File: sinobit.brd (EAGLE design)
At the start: 92 x 92.1 mm, 254 parts, among them J1 TWIG_2.0, J2 TWIG_2.0, U1 SPX3819, U10 16MHZ2520, U6 IC_NRF51822_MODULE, U8 HT1632C_QFP52, U9 16MHZ2520

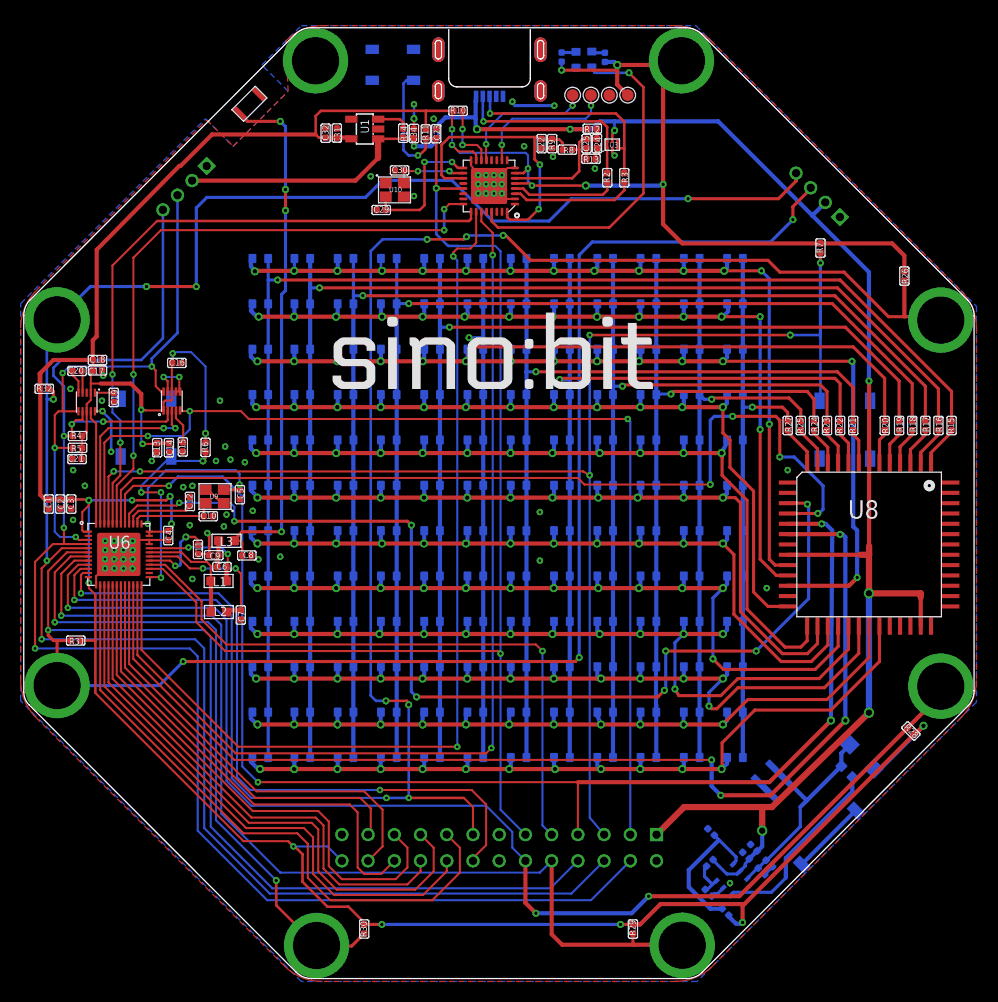
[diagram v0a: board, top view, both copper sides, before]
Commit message: sinobit-V1.0
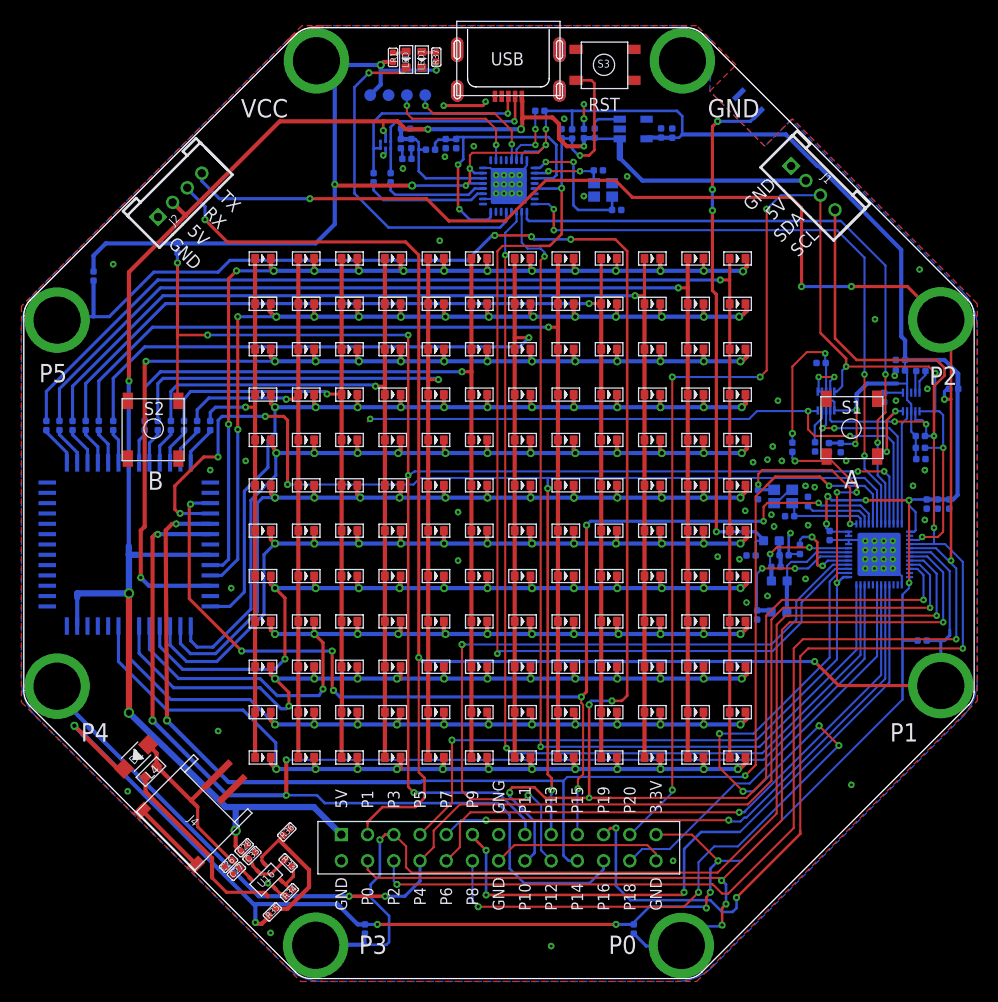
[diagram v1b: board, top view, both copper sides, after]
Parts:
- removed U$1: (no value), Logo:SINOBIT3
- removed U$13: IC_MMA8653FCR1, mirco：bit:MMA8653FC
- removed U$4: PS7516, microbit2:PS7516
- removed U$6: TIANXIAN, microbit2:TIANXIAN
- removed U$7: IC_MKL26Z128VFM4, Modulebit_open_Eagle:MKL26Z168VFM4
- added E$1: (no value), XZX1:文字
- added E$2: (no value), XZX:SINOBIT2
- added E$3: (no value), XZX1:ELECEOW
- added E$4: (no value), XZX:SINOBIT编号
- added E$5: (no value), XZX:XXX
- added U11: TIANXIAN, microbit2:TIANXIAN
- added U12: IC_MKL26Z128VFM4, Modulebit_open_Eagle:MKL26Z168VFM4
- added U14: IC_MMA8653FCR1, mirco：bit:MMA8653FC
- added U16: PS7516, microbit2:PS7516
- C33: value 22uF -> 10uF
- R26, R28, R29, R30, R31, R32: value 3.3M -> 2M
- R33: value 525K -> 510k
- moved R32 88.1 mm to (77.4, 30.1), flipped to the bottom
- moved R15 87.7 mm to (-10.5, 26.5), flipped to the bottom
- moved C1 87.2 mm to (77.0, 18.9), flipped to the bottom
- moved U$35 85.6 mm to (76.2, 1.36), flipped to the bottom
- moved U$39 85.6 mm to (76.2, 36.8), flipped to the bottom
- moved U$48 85.6 mm to (-9.42, 36.8), flipped to the bottom
- moved U$49 85.6 mm to (-9.42, 1.30), flipped to the bottom
- moved R16 85.1 mm to (-9.19, 26.5), flipped to the bottom
- moved C2 85.0 mm to (75.9, 18.9), flipped to the bottom
- moved C3 82.9 mm to (74.8, 18.9), flipped to the bottom
- moved R17 82.6 mm to (-7.92, 26.5), flipped to the bottom
- moved R31 82.0 mm to (74.4, 5.71), flipped to the bottom
- moved C20 81.7 mm to (74.2, 31.8), flipped to the bottom
- moved C21 81.7 mm to (74.2, 23.3), flipped to the bottom
- moved R4 81.6 mm to (74.2, 25.5), flipped to the bottom
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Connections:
- removed net N$7: R30.2, U$51.P$1, U6.7
- removed net P0.8: U$12.P$9, U6.14
- new net P0.3: R30.2, U$12.P$25, U$51.P$1, U6.7
- net 3.3V: now also U$12.P$13, U12.15, U12.5, U12.7, U14.8, U14.P1; no longer U$12.P$14, U$13.8, U$13.P1, U$7.15, U$7.5, U$7.7
- net 8653_INT1: now also U14.P3; no longer U$13.P3
- net 8653_INT2: now also U14.P5; no longer U$12.P$2, U$13.P5
- net BTN_A: now also U$12.P$4
- net BTN_B: now also U$12.P$8; no longer U$12.P$3
- net GND: now also U$12.P$14, U12.16, U12.2, U12.8, U14.6, U14.7, U14.9, U16.P2; no longer U$12.P$13, U$13.6, U$13.7, U$13.9, U$4.P2, U$7.16, U$7.2, U$7.8
- net MISO: now also U$12.P$17; no longer U$12.P$4
- net MOSI: now also U$12.P$10
- net N$11: now also U12.29; no longer U$7.29
- net N$14: now also U12.3; no longer U$7.3
- net N$15: now also U12.4; no longer U$7.4
- net N$16: now also U12.17; no longer U$7.17
- net N$17: now also U12.18; no longer U$7.18
- net N$18: now also U16.P4; no longer U$4.P4
- net N$19: now also U16.P6; no longer U$4.P6
- net N$22: now also U16.P1; no longer U$4.P1
- net N$23: now also U11.P$1; no longer U$6.P$1
- net N$26: now also U16.P3; no longer U$4.P3
- net N$3: now also U12.14; no longer U$7.14
- net N$4: now also U14.P4; no longer U$13.P4
- net N$8: now also U12.10; no longer U$7.10
- net N$9: now also U12.13; no longer U$7.13
- net P0.10: now also U$12.P$6; no longer U$12.P$10
- net P0.11: now also U$12.P$5; no longer U$12.P$17
- net P0.12: now also U$12.P$22; no longer U$12.P$11
- net P0.13: now also U$12.P$15; no longer U$12.P$16
- net P0.14: no longer U$12.P$12
- net P0.15: no longer U$12.P$15
- net P0.16: now also U$12.P$16
- net P0.18: now also U$12.P$21
- net P0.2/RX: now also U$12.P$2; no longer U$12.P$23
- net P0.20: now also U$12.P$18; no longer U$12.P$5
- net P0.4: now also U$12.P$3; no longer U$12.P$22
- net P0.5: now also U$12.P$23; no longer U$12.P$21
- net P0.6: now also U$12.P$19; no longer U$12.P$8
- net P0.7: no longer U$12.P$19
- net P0.9: no longer U$12.P$18
- net RST: now also U12.19, U12.32; no longer U$7.19, U$7.32
- net RX: now also U12.25; no longer U$7.25
- net SCK: now also U$12.P$9
- net SCL: now also U$12.P$11, U14.P2; no longer U$12.P$25, U$13.P2
- net SDA: now also U$12.P$12, U14.10; no longer U$13.10
- net TGT_NRESET: now also U12.21; no longer U$12.P$6, U$7.21
- net TGT_SWCLK: now also U12.26; no longer U$7.26
- net TGT_SWDIO: now also U12.27; no longer U$7.27
- net TX: now also U12.24; no longer U$7.24
- net VCC: now also U16.P5; no longer U$4.P5
- net VCC1: now also U12.6; no longer U$7.6
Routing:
- net P0.3: track 0.00 -> 101.6 mm, vias 0 -> 4
- net P0.18: track 0.00 -> 90.4 mm, vias 0 -> 6
- net SDA: track 52.4 -> 129.3 mm, vias 4 -> 8
- net P0.7: track 65.6 -> 0.00 mm, vias 2 -> 0
- net N$7: track 64.5 -> 0.00 mm, vias 2 -> 0
- net P0.8: track 60.7 -> 0.00 mm
- net BTN_A: track 20.7 -> 79.8 mm, vias 4 -> 5
- net P0.9: track 55.4 -> 0.00 mm
- net P0.2/RX: track 208.0 -> 156.0 mm, vias 4 -> 3
- net P0.15: track 43.6 -> 0.00 mm
- net P0.14: track 40.1 -> 0.00 mm
- net 8653_INT2: track 102.5 -> 62.5 mm
- net P0.16: track 109.6 -> 148.8 mm
- net SCK: track 89.2 -> 123.9 mm, vias 4 -> 6
- net TGT_NRESET: track 127.1 -> 109.4 mm
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- added copper zone on layer 1, net N$10
- removed copper zone on layer 16, net N$10
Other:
- outline, holes or cut-outs redrawn
- board text added: "3.3V"
- board text added: "GNG"
- board text added: "P10"
- board text added: "P11"
- board text added: "P12"
- board text added: "P13"
- board text added: "P14"
- board text added: "P15"
- board text added: "P16"
- board text added: "P18"
- board text added: "P19"
- board text added: "P20"
- board text added: "P6"
- board text added: "P7"
- board text added: "P8"
- board text added: "P9"
- board text added: "RST"
- board text added: "U11"
- board text added: "U12"
- board text added: "U14"
- board text added: "U16"
